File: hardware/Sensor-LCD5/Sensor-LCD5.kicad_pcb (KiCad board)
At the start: 2 copper layers, 83.8 x 20.3 mm, 19 parts, among them Q1 TEPT5700, Q2 TEPT5700, Q3 TEPT5700, Q4 TEPT5700, Q5 TEPT5700, U1 MCP6002-xMC, U2 MCP6002-xMC, U3 MCP6002-xMC, U4 PIC32CM PL10

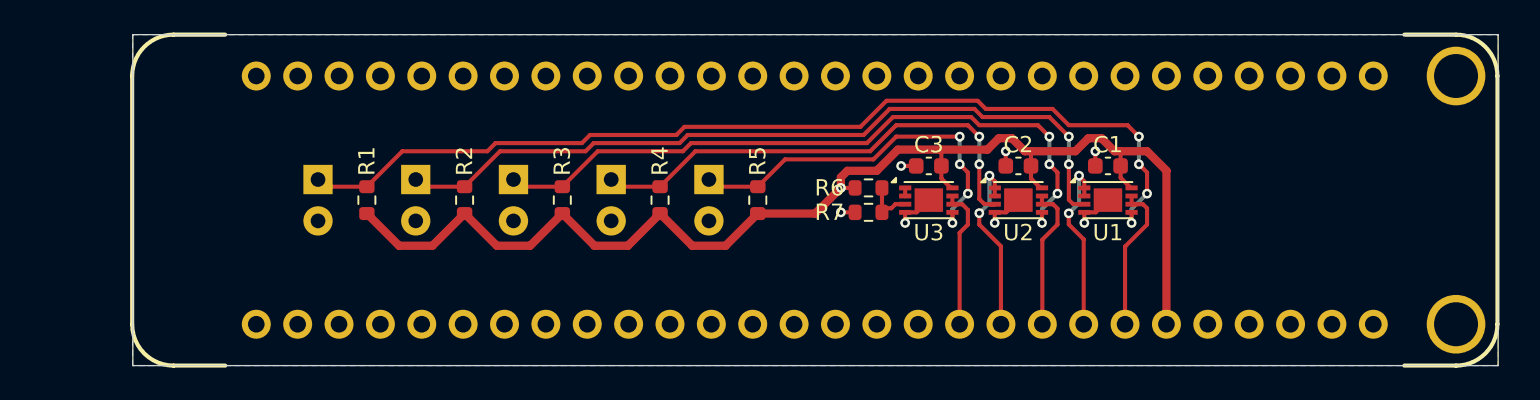
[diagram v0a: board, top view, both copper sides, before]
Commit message: work on sensor board
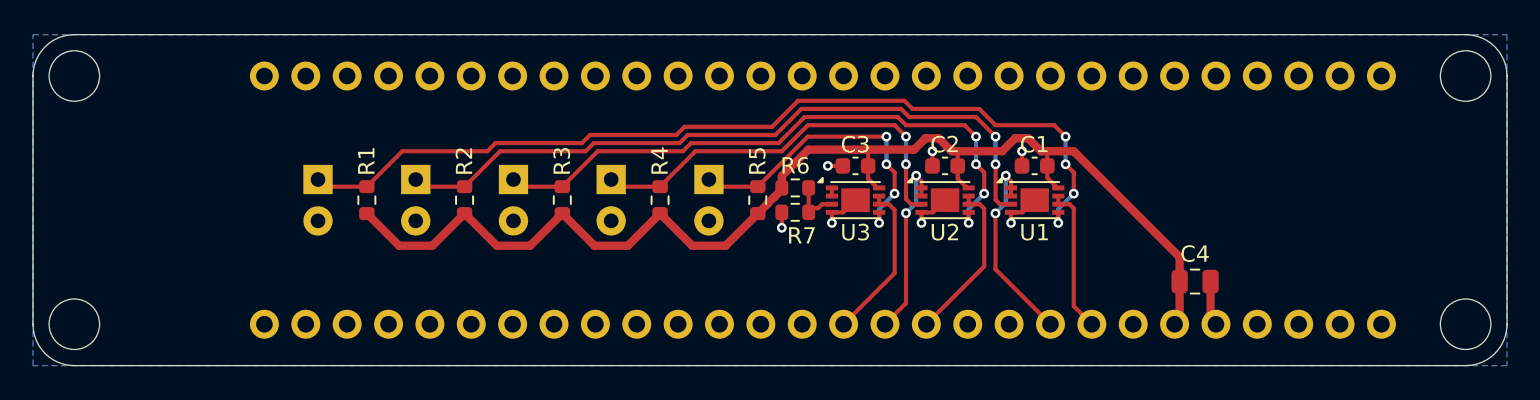
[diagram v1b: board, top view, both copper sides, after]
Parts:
- added C4: 10uF, Capacitor_SMD:C_0805_2012Metric, F.Cu at (153.8, 105.0)
- moved C1 4.50 mm to (144.0, 97.9)
- moved C2 4.50 mm to (138.5, 97.9)
- moved C3 4.50 mm to (133.0, 97.9)
- moved R6 4.50 mm to (129.3, 99.2)
- moved R7 4.50 mm to (129.3, 100.8)
- moved U1 4.50 mm to (144.0, 100.0)
- moved U2 4.50 mm to (138.5, 100.0)
- moved U3 4.50 mm to (133.0, 100.0)
- moved U4 0.50 mm to (131.0, 100.0)
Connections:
- U4 pad 43: unconnected-(U4-ADC_0-Pad43) -> /TRACK_ORANGE
- U4 pad 44: unconnected-(U4-ADC_1-Pad44) -> /TRACK_BLUE
- U4 pad 45: unconnected-(U4-ADC_2-Pad45) -> /TRACK_YELLOW
- U4 pad 46: /TRACK_ORANGE -> unconnected-(U4-PWM_3-Pad46)
- U4 pad 47: /TRACK_BLUE -> unconnected-(U4-PWM_4-Pad47)
- U4 pad 48: /TRACK_YELLOW -> /TRACK_RED
- U4 pad 49: /TRACK_RED -> /TRACK_GREEN
- U4 pad 50: /TRACK_GREEN -> unconnected-(U4-ADC_7-Pad50)
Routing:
- net Net-(Q2-C): track 47.9 -> 43.4 mm
- net Net-(Q4-C): track 29.8 -> 25.3 mm
- net Net-(Q1-C): track 60.2 -> 55.7 mm
- net Net-(Q5-C): track 23.4 -> 18.9 mm
- net Net-(Q3-C): track 41.9 -> 37.4 mm
- net VCC: track 77.6 -> 74.7 mm, vias 1 -> 0
- net COM: track 10.8 -> 13.7 mm
- net /TRACK_YELLOW: track 9.05 -> 10.1 mm
- net /TRACK_ORANGE: track 8.83 -> 9.91 mm
- net /TRACK_RED: track 11.2 -> 12.2 mm
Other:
- board size 83.8 x 20.3 mm -> 90.5 x 20.3 mm
